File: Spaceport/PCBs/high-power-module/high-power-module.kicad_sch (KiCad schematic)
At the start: 76 parts, among them J1 Conn_01x06_Pin, J2 SMA, J3 Conn_01x06_Pin, J4 Conn_01x02_Pin, U1 Si4463, U2 SN74LV1T08QDBVRQ1, U3 TPS62177DQCR

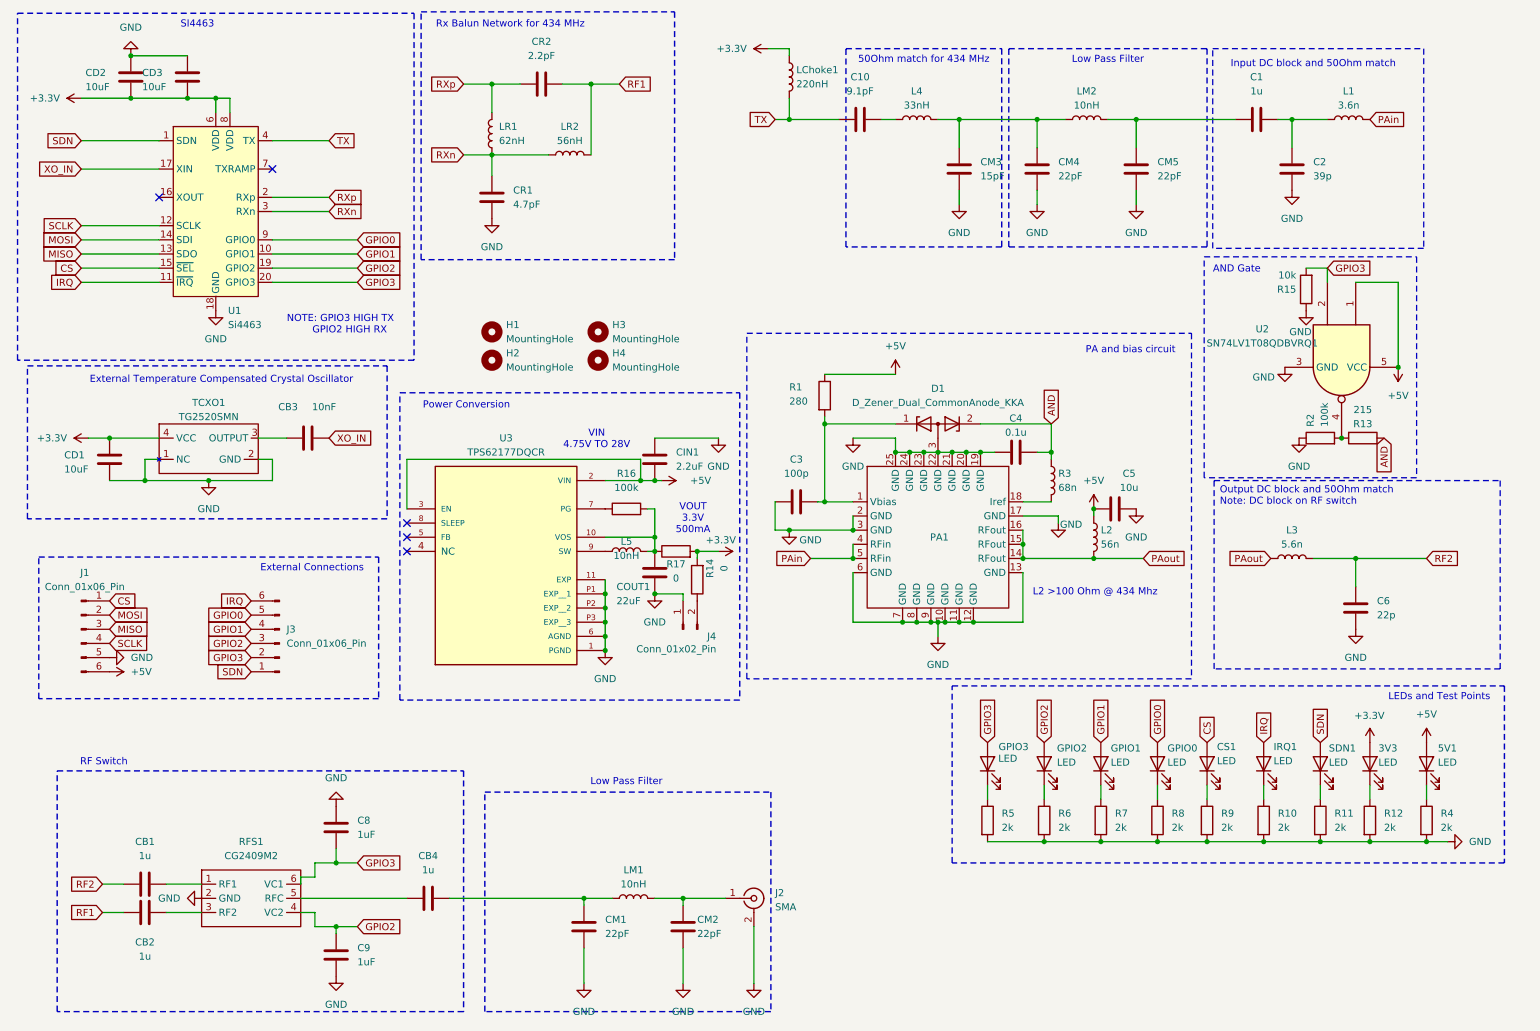
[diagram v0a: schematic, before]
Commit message: update HPM based on sims
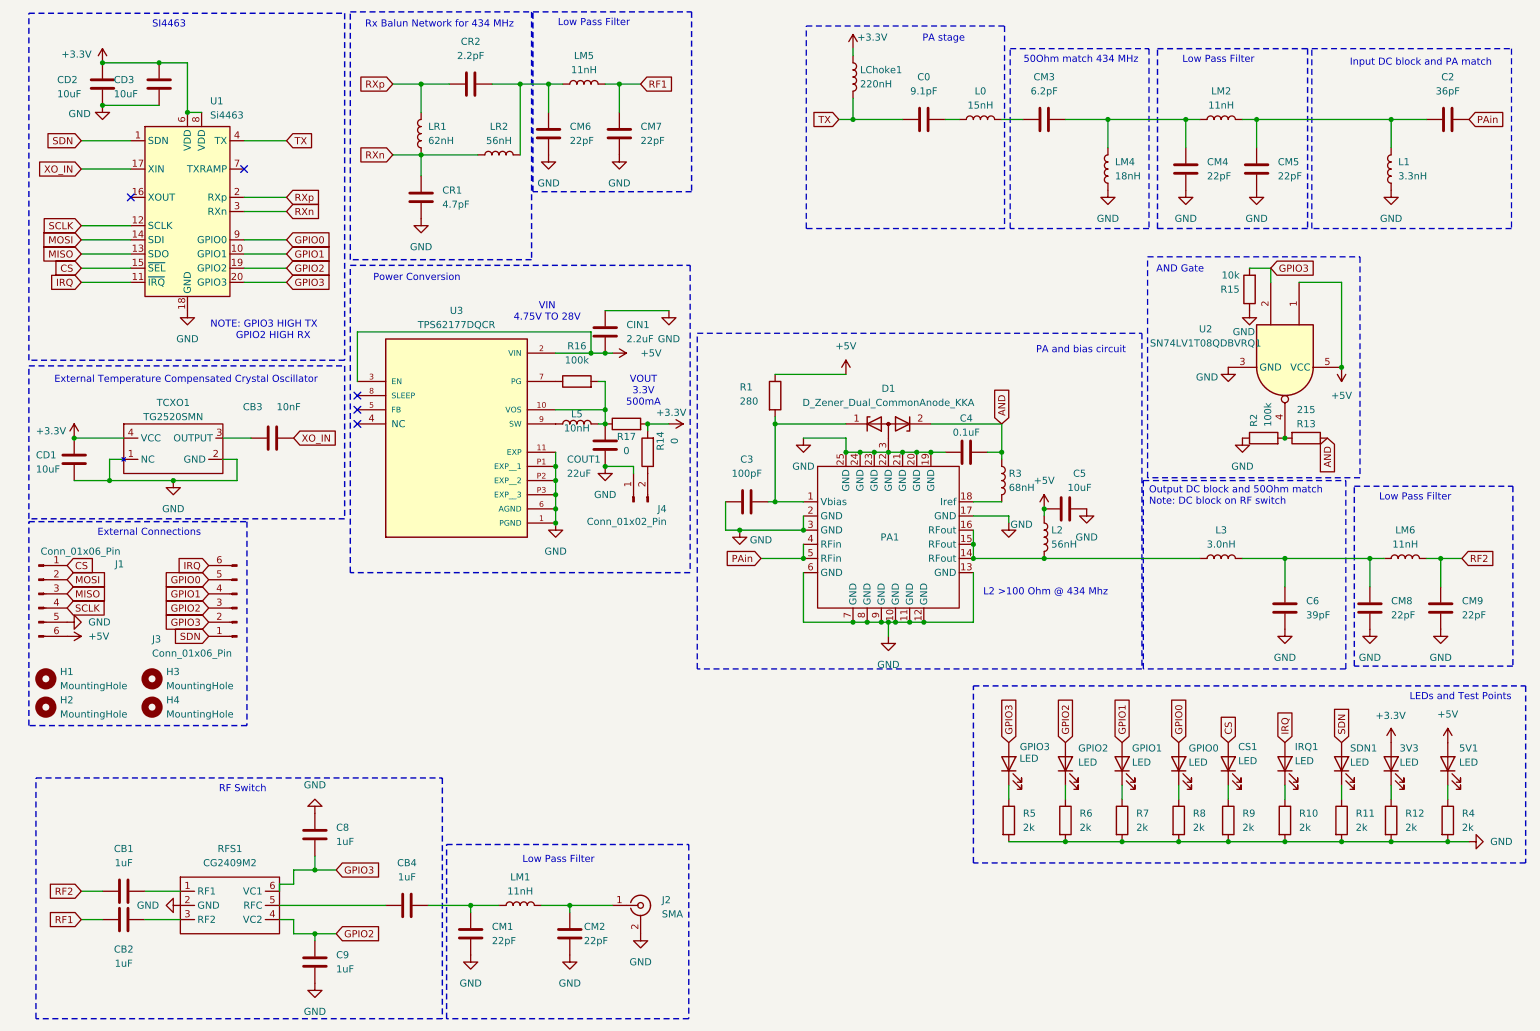
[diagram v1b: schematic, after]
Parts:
- removed C1: 1u, Capacitor_SMD:C_0805_2012Metric_Pad1.18x1.45mm_HandSolder, symbol Device:C
- removed L4: 33nH, Inductor_SMD:L_0805_2012Metric_Pad1.15x1.40mm_HandSolder, symbol Device:L
- added CM6, CM7, CM8, CM9: 22pF, Capacitor_SMD:C_0805_2012Metric_Pad1.18x1.45mm_HandSolder, symbol Device:C
- added L0: 15nH, Inductor_SMD:L_0805_2012Metric_Pad1.15x1.40mm_HandSolder, symbol Device:L
- added LM4: 18nH, Inductor_SMD:L_0805_2012Metric_Pad1.15x1.40mm_HandSolder, symbol Device:L
- added LM5, LM6: 11nH, Inductor_SMD:L_0805_2012Metric_Pad1.15x1.40mm_HandSolder, symbol Device:L
- C2: value 39p -> 36pF
- C3: value 100p -> 100pF
- C4: value 0.1u -> 0.1uF
- C5: value 10u -> 10uF
- C6: value 22p -> 39pF
- CB1, CB2, CB4: value 1u -> 1uF
- CM3: value 15pF -> 6.2pF
- L1: value 3.6n -> 3.3nH
- L2: value 56n -> 56nH
- L3: value 5.6n -> 3.0nH
- LM1, LM2: value 10nH -> 11nH
- R3: value 68n -> 68nH
- renumbered C10 to C0
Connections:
- net +3.3V: now also CD2.1, CD3.1; no longer CD2.2, CD3.2
- net GND: now also CD2.2, CD3.2, L1.1, CM6.2, CM7.2, CM8.2, CM9.2, LM4.1; no longer C2.1, CD2.1, CD3.1, CM3.2
- net PAin: now also C2.1; no longer L1.2
- net RF1: now also CM7.1, LM5.2; no longer CR2.2, LR2.2
- net RF2: now also CM9.1, LM6.2; no longer C6.2, L3.2
- net at CM4.1, LM2.1: now also CM3.2, LM4.2; no longer CM3.1
- net at C0.2: now also L0.1
- net at C2.2: now also CM5.1, L1.2, LM2.2; no longer L1.1
- net PAout: no longer names the net of L2.2, L3.1, PA1.14 (RFout), PA1.15 (RFout), PA1.16 (RFout)
- new net: CM3.1, L0.2
- new net: CM6.1, CR2.2, LM5.1, LR2.2
- new net: C6.2, CM8.1, L3.2, LM6.1
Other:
- note added: "50Ohm match 434 MHz"
- note added: "Input DC block and PA match"
- note added: "PA stage"
- note removed: "50Ohm match for 434 MHz"
- note removed: "Input DC block and 50Ohm match"
- moved on the sheet: 3V3, 5V1, C0, C2, C3, C4, C5, C6, C8, C9, CB1, CB2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
